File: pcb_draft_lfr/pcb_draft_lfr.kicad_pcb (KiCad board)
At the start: 2 copper layers, 54.8 x 64.6 mm, 50 parts, among them J1 Conn_01x03_Pin, J10 Conn_01x02_Pin, J2 Conn_01x03_Pin, J3 Conn_01x03_Pin, J4 Conn_01x03_Pin, J5 Conn_01x03_Pin, J6 Conn_01x02_Pin, J7 Conn_01x02_Pin, J8 Conn_01x04_Pin, J9 AVR-ISP-6, Q1 MOSFET N-Channel, Q2 MOSFET N-Channel, U1 Voltage Regulator, U2 ATMEGA328-PU, X1 Crystal SMD

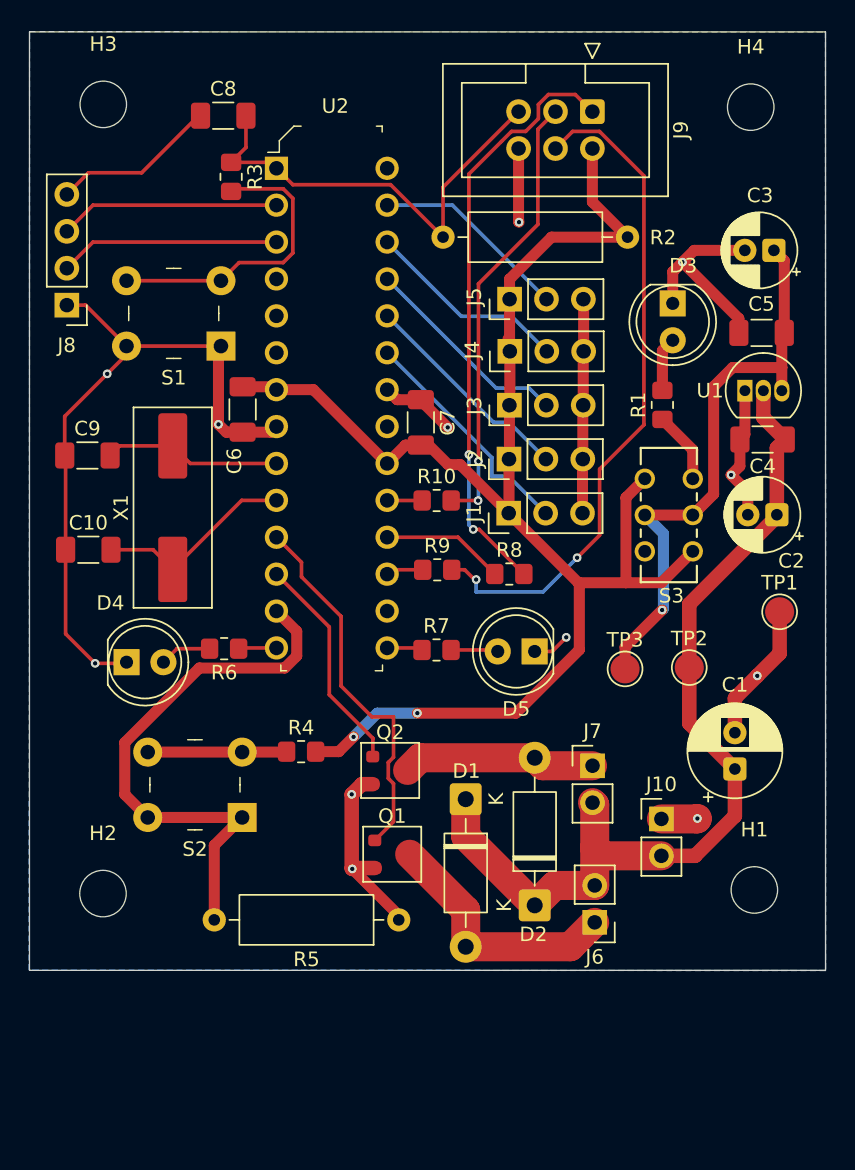
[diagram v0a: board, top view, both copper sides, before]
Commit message: REV3/4
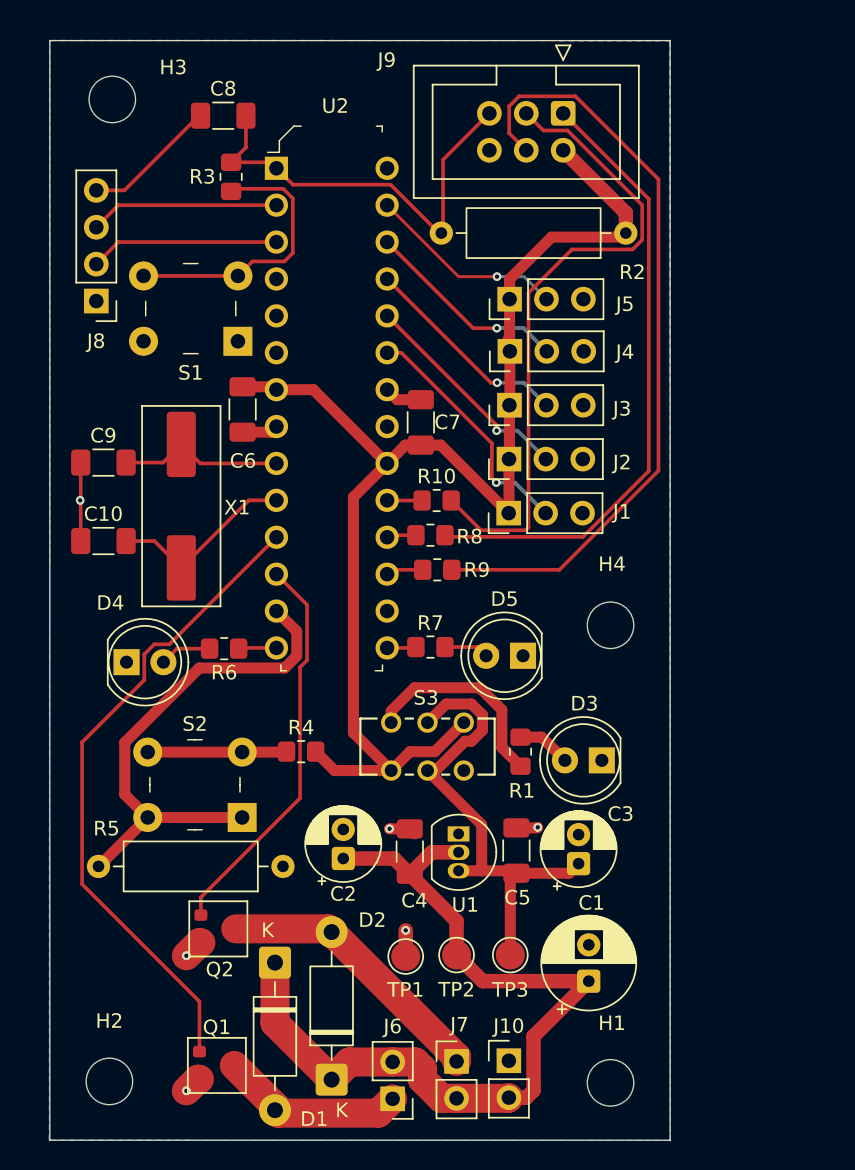
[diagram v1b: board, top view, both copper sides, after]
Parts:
- moved C3 44.3 mm to (137.9, 131.0), turned to 90 degrees
- moved C5 39.4 mm to (133.6, 130.1), turned to 90 degrees
- moved C2 38.1 mm to (121.7, 130.7), turned to 90 degrees
- moved C4 37.3 mm to (126.3, 130.2), turned to 90 degrees
- moved H4 37.0 mm to (140.1, 114.6)
- moved U1 36.3 mm to (129.6, 129.0), turned to -90 degrees
- moved TP1 35.0 mm to (126.0, 137.4)
- moved D3 31.8 mm to (139.5, 123.9), turned to 180 degrees
- moved S3 26.6 mm to (125.0, 124.6), turned to 90 degrees
- moved R1 25.8 mm to (133.9, 123.3)
- moved TP2 25.5 mm to (129.5, 137.3)
- moved J7 22.4 mm to (129.5, 144.6)
- moved TP3 21.2 mm to (133.2, 137.3)
- moved J10 19.7 mm to (133.1, 144.6)
- moved Q1 18.9 mm to (113.0, 144.9)
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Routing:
- net GND: track 125.2 -> 19.2 mm, vias 12 -> 6
- net Vgate1: track 25.9 -> 44.9 mm
- net Net-(J9-SCK): track 30.8 -> 44.7 mm, vias 2 -> 0
- net Vcc: track 104.7 -> 91.4 mm, vias 2 -> 0
- net Vgate2: track 15.3 -> 27.4 mm
- net Net-(R1-+): track 4.95 -> 14.1 mm
- net Net-(J9-MOSI): track 46.8 -> 53.6 mm, vias 2 -> 0
- net Net-(U1-VO): track 40.2 -> 33.5 mm, vias 1 -> 0
- net Vmiso: track 8.64 -> 2.04 mm
- net Net-(D2-A): track 13.3 -> 19.2 mm
- net Vbat+: track 65.3 -> 60.6 mm
- net Net-(D1-A): track 17.5 -> 12.8 mm
- net Button1: track 38.1 -> 35.1 mm
- net TXD: track 15.2 -> 13.0 mm
- net RXD: track 15.2 -> 13.0 mm
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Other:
- board size 54.8 x 64.6 mm -> 42.7 x 75.7 mm
